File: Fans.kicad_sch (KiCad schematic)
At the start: 20 parts, among them Q1 PSMN8R5-40MSDX, Q2 PSMN8R5-40MSDX, U2 EMC2305-1-AP-TR

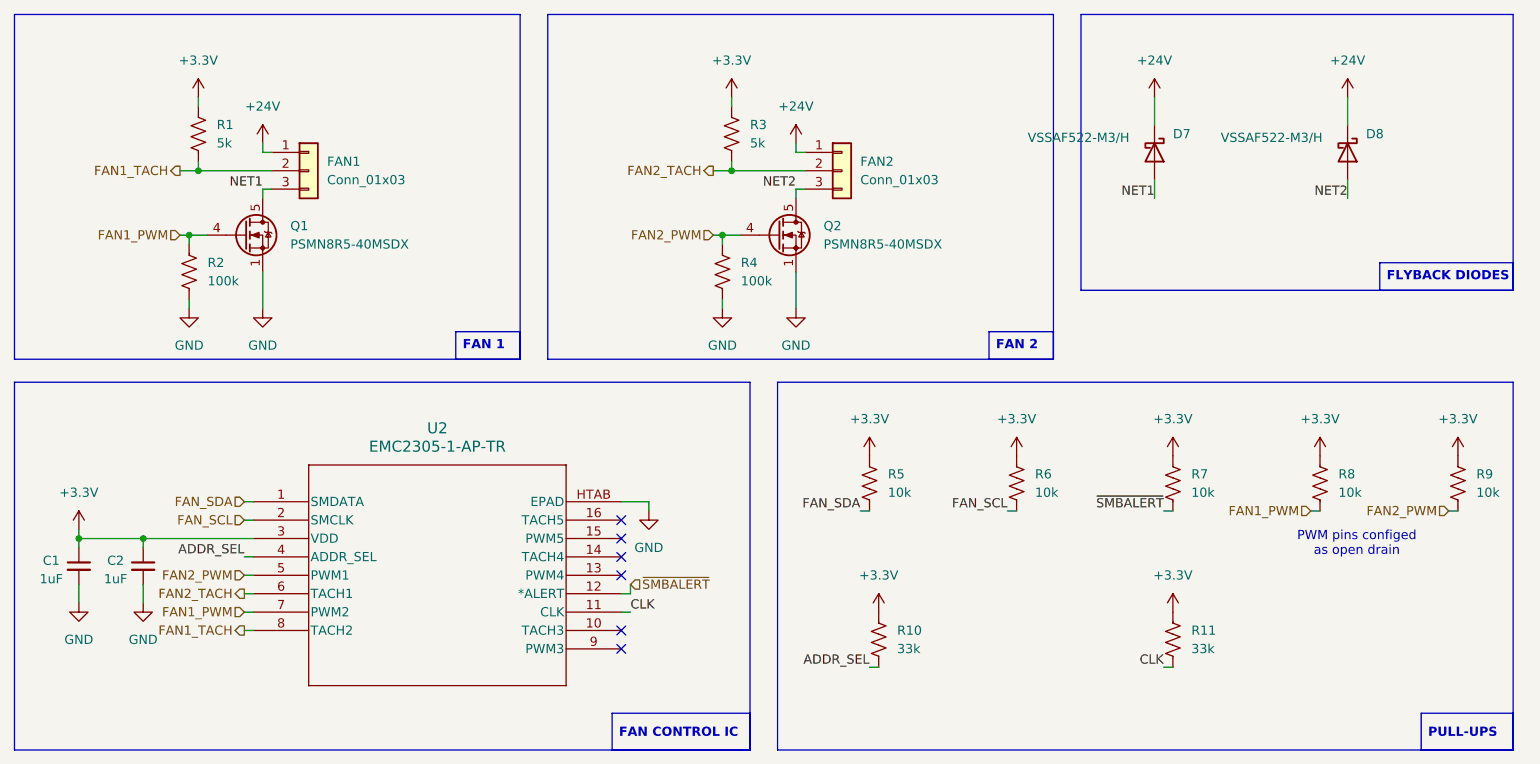
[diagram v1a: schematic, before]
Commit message: fixed cap vals + made schem pretty
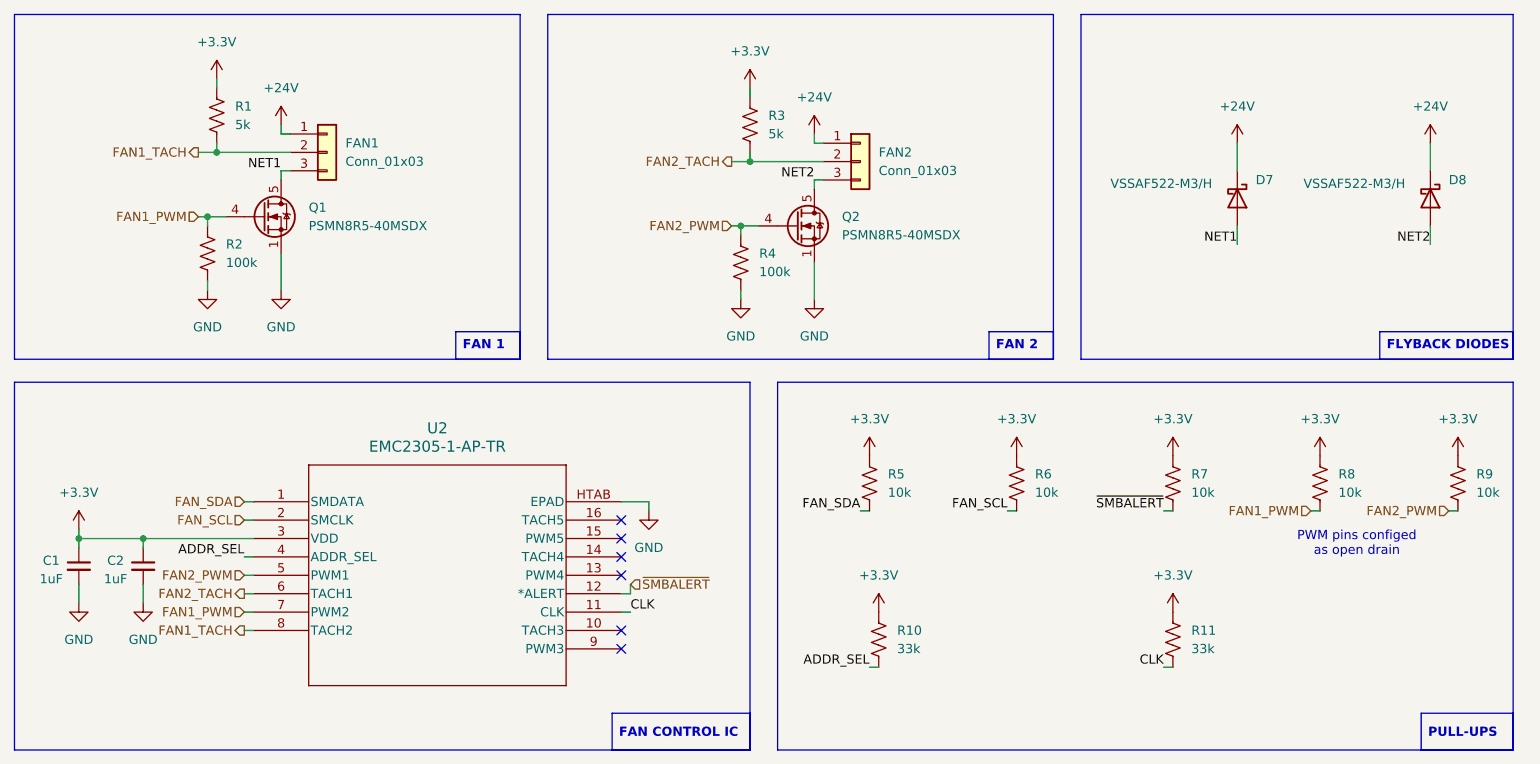
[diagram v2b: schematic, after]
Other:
- moved on the sheet: D7, D8, FAN1, FAN2, Q1, Q2, R1, R2, R3, R4

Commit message: initial schem changes
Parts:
- D7, D8: footprint UTSVT_Passive:MMDL101T1G -> Package_TO_SOT_THT:TO-247-2_Vertical
